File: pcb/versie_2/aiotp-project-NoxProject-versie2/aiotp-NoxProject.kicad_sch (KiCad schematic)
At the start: 9 parts, among them J2 GPS connector, J3 Stemma connector, U1 DFR0478

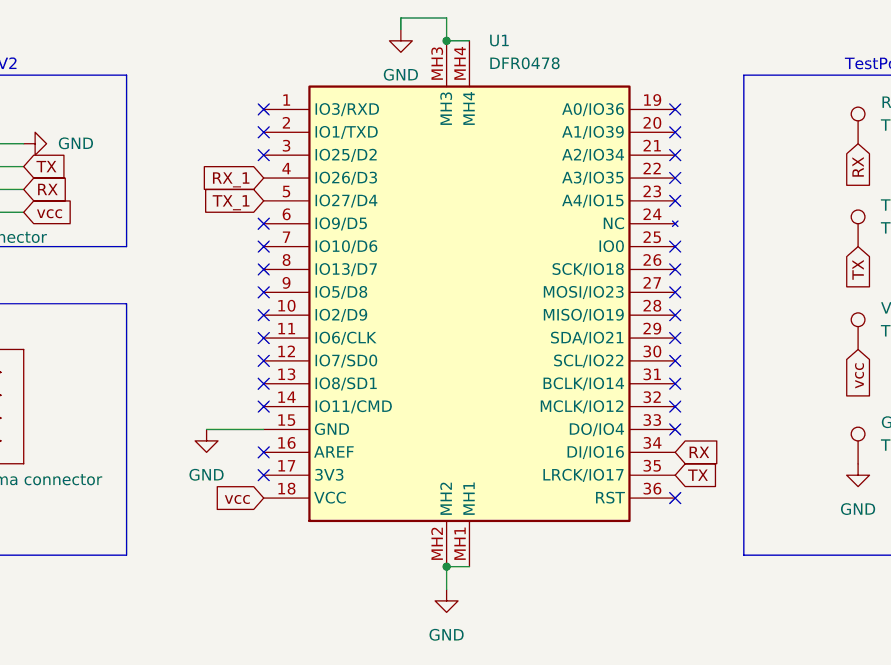
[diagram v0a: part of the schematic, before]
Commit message: PCB en influx en node
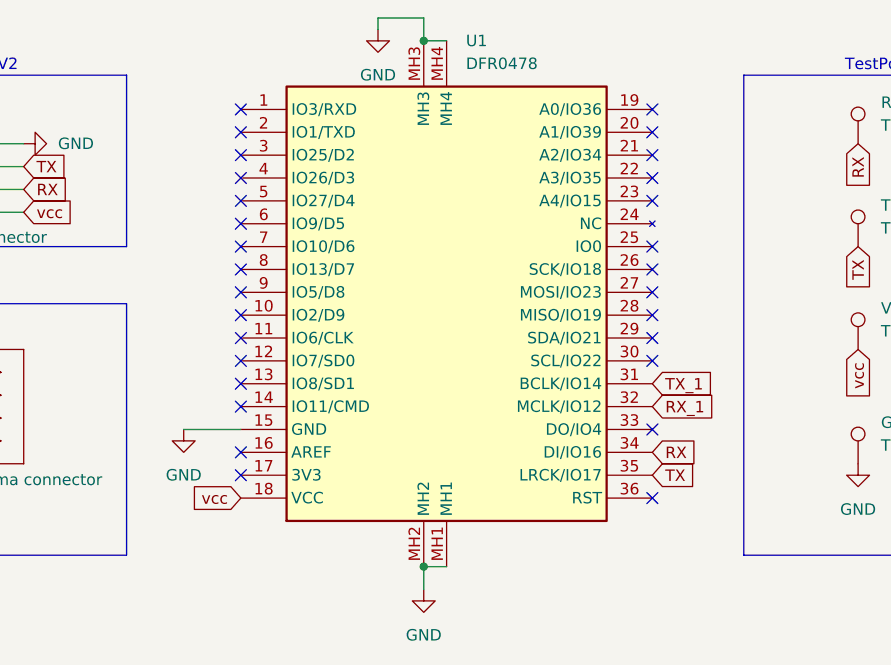
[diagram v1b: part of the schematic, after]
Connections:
- net RX_1: now also U1.32 (MCLK/IO12); no longer U1.4 (IO26/D3)
- net TX_1: now also U1.31 (BCLK/IO14); no longer U1.5 (IO27/D4)
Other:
- moved on the sheet: U1

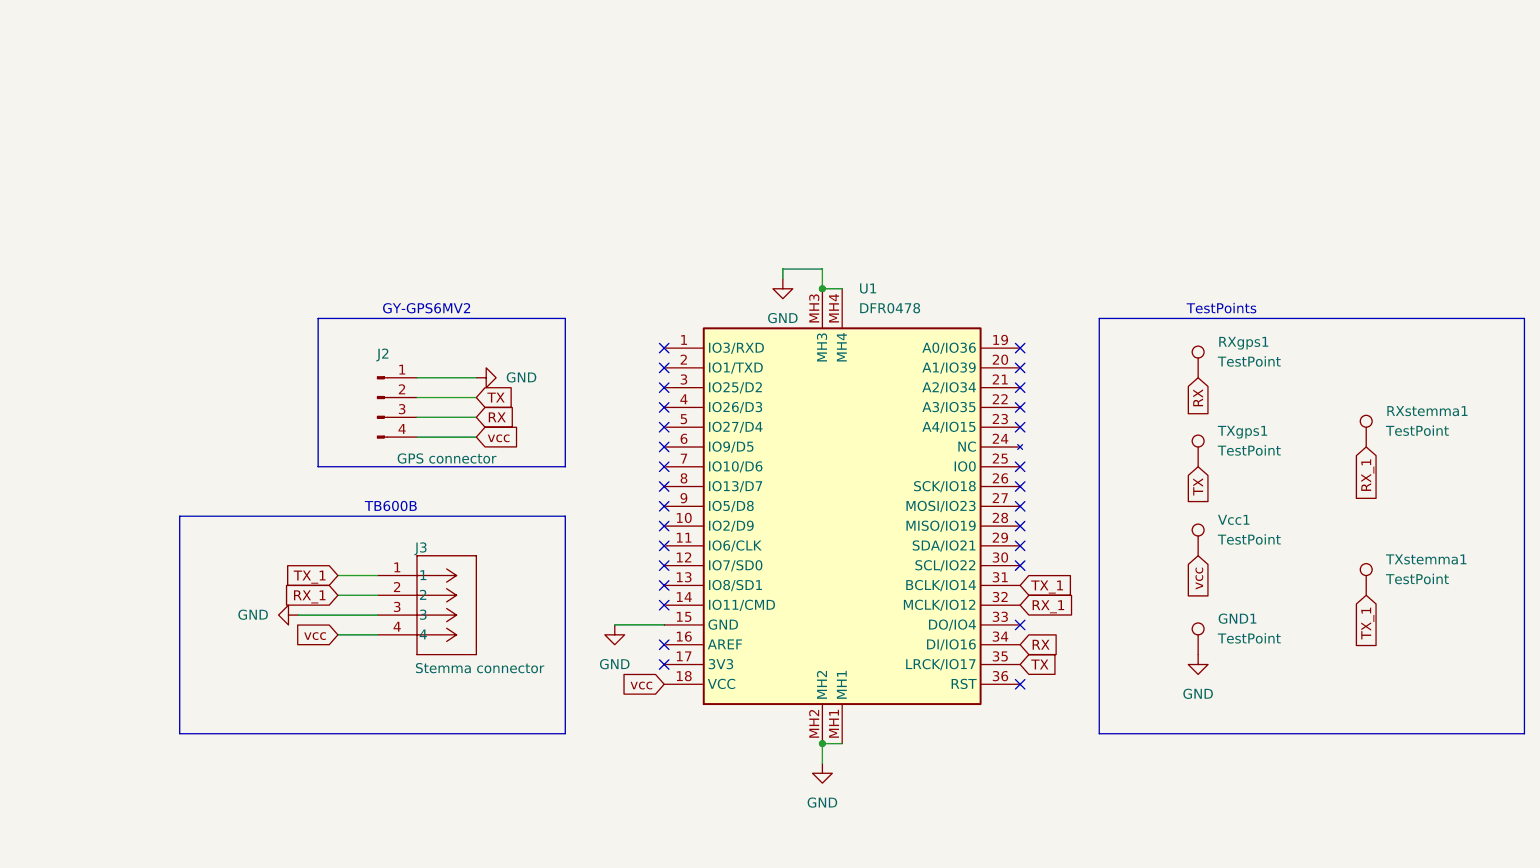
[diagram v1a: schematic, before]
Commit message: pcb
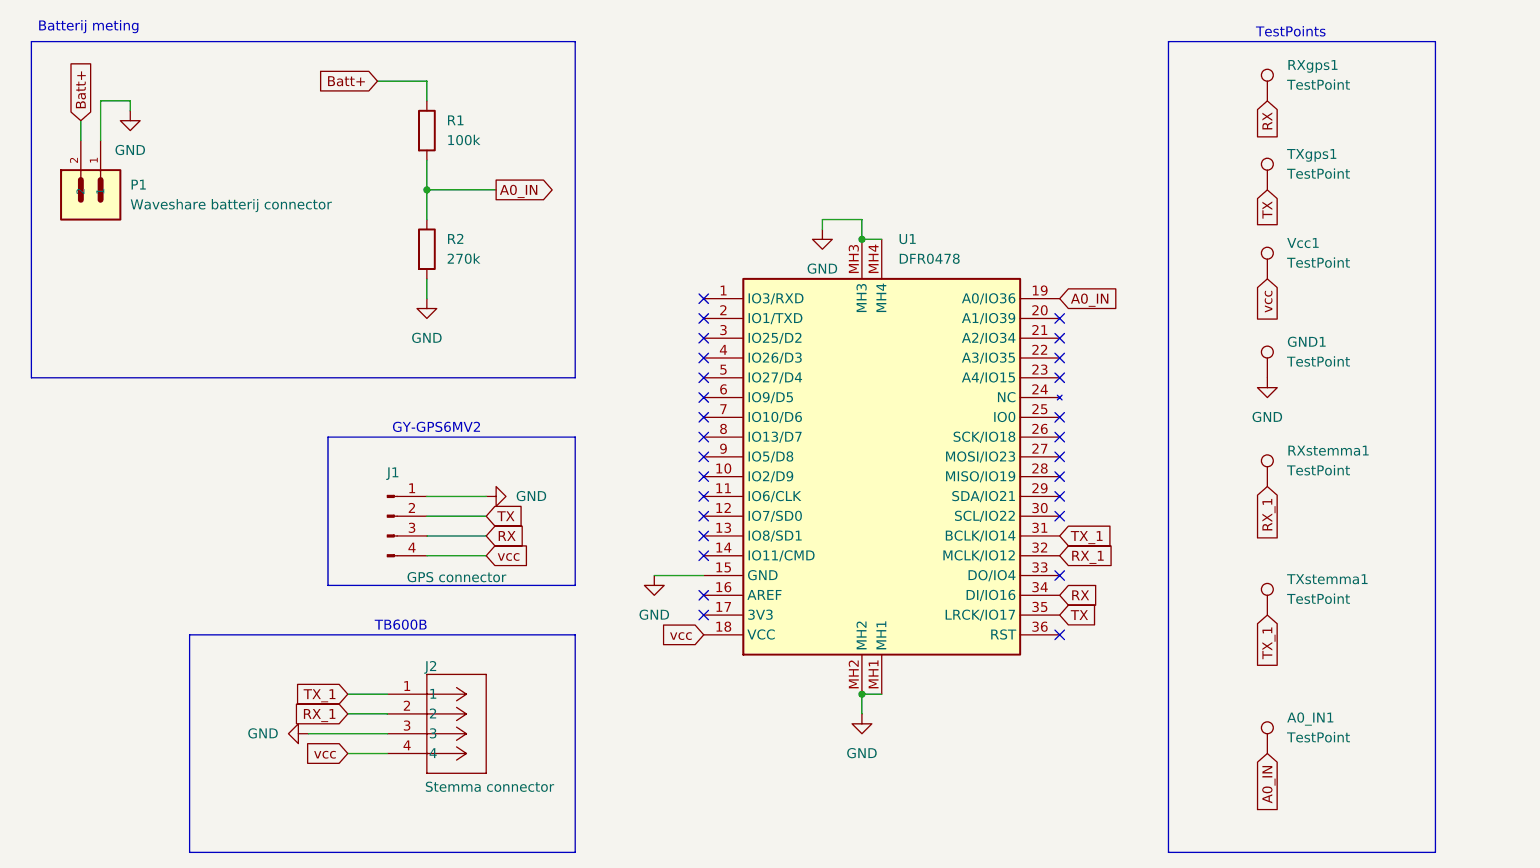
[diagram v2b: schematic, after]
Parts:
- added A0_IN1: TestPoint, TestPoint:TestPoint_THTPad_D1.0mm_Drill0.5mm, symbol Connector:TestPoint
- added P1: Waveshare batterij connector, Library:JST_S2B-PH-SM4-TB, symbol footprints:S2B-PH-SM4-TB
- added R1: 100k, Resistor_SMD:R_0805_2012Metric, symbol Device:R
- added R2: 270k, Resistor_SMD:R_0805_2012Metric, symbol Device:R
- renumbered J2 to J1, J3 to J2
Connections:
- net GND: now also P1.1, R2.2
- net A0_IN: now reaches U1.19 (A0/IO36)
- net A0_IN: now also A0_IN1.1, R1.2, R2.1
- new net Batt+: P1.2, R1.1
- no-connect marks 29 -> 28
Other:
- note added: "Batterij meting"
- moved on the sheet: GND1, J1, J2, RXgps1, RXstemma1, TXgps1, TXstemma1, U1, Vcc1
